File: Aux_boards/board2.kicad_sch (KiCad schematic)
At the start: 30 parts, among them J1 DA15_Plug_MountingHoles, U2 AMS1117-3.3, U3 SFH6345, U4 SFH6345, U5 SFH6345, U6 SFH6345, U7 SFH6345, U8 SFH6345, U9 SFH6345

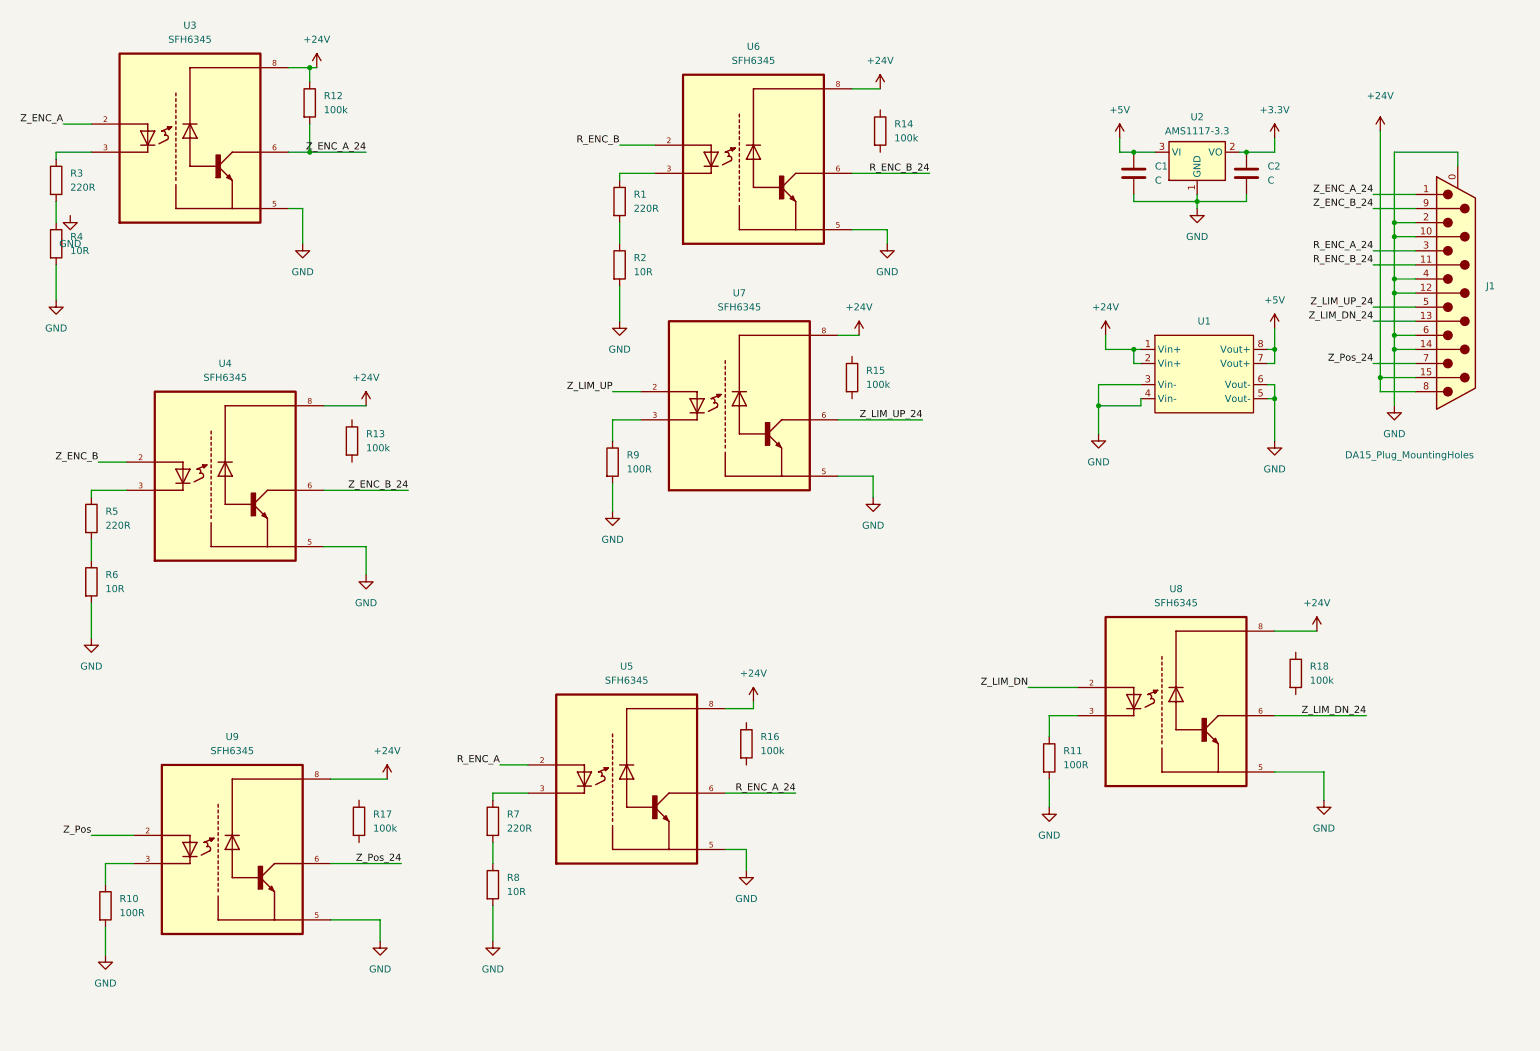
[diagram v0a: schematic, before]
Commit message: jeee
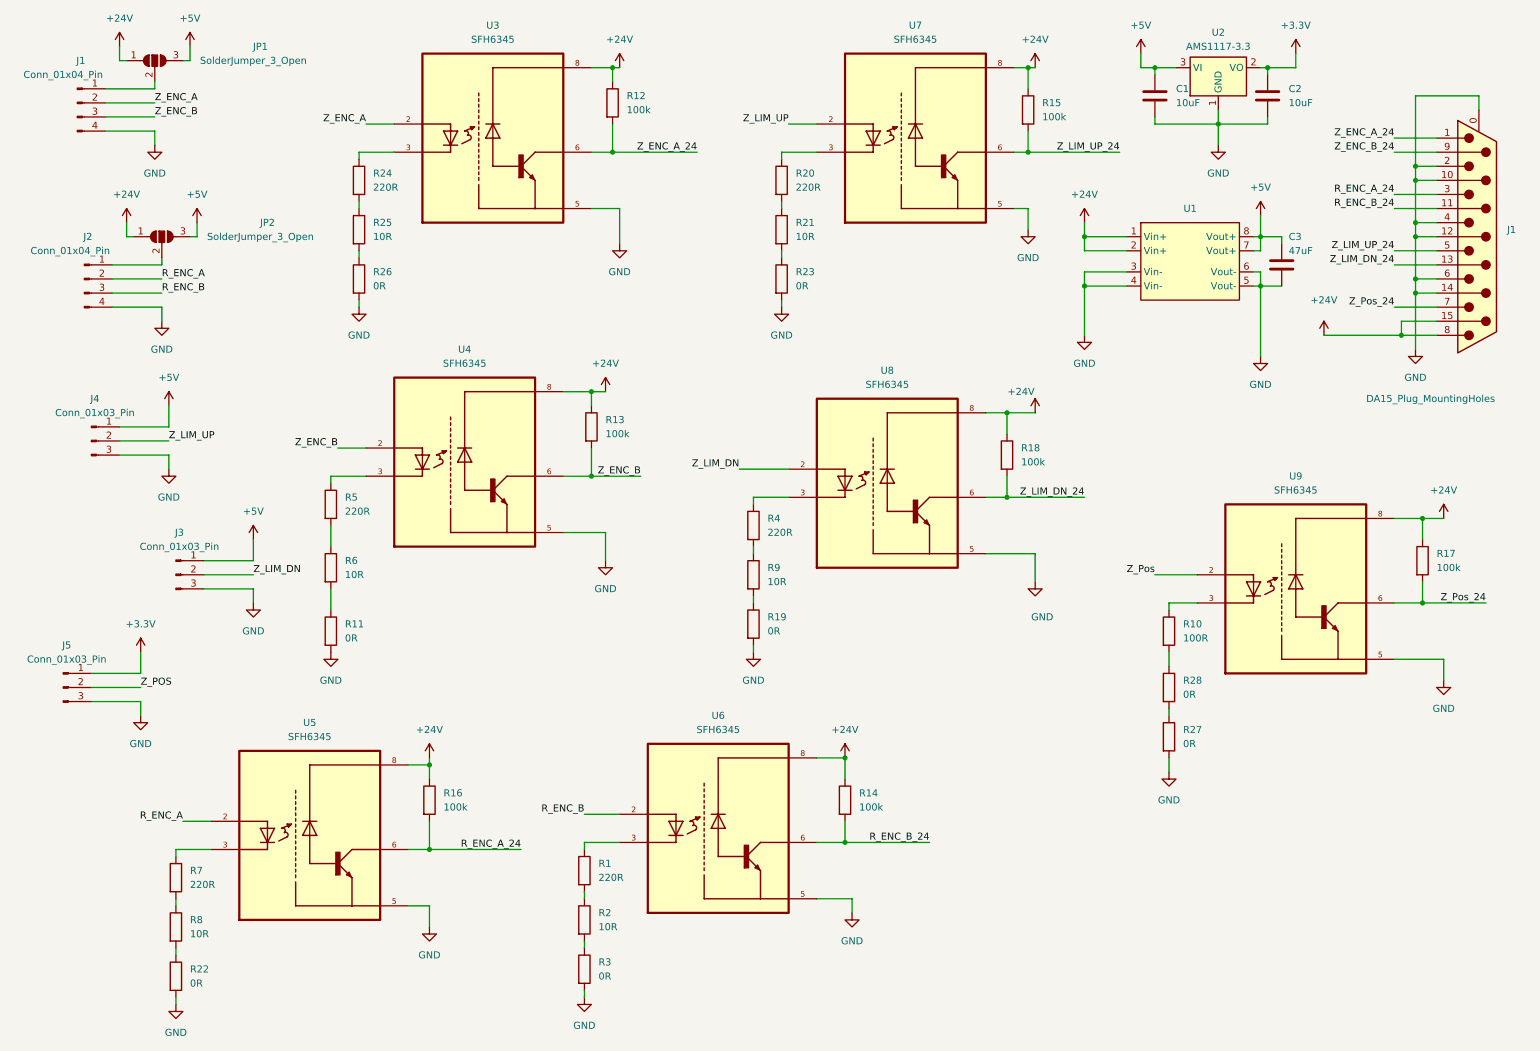
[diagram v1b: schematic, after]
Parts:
- added C3: 47uF, symbol Device:C
- added J1, J2: Conn_01x04_Pin, symbol Connector:Conn_01x04_Pin
- added J3, J4, J5: Conn_01x03_Pin, symbol Connector:Conn_01x03_Pin
- added JP1, JP2: SolderJumper_3_Open, symbol Jumper:SolderJumper_3_Open
- added R19, R22, R23, R26, R27, R28: 0R, symbol Device:R
- added R20, R24: 220R, symbol Device:R
- added R21, R25: 10R, symbol Device:R
- C1, C2: value C -> 10uF
- R11: value 100R -> 0R
- R3: value 220R -> 0R
- R4: value 10R -> 220R
- R9: value 100R -> 10R
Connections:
- net +24V: now also R13.1, R14.1, R15.1, R16.1, R17.1, R18.1, JP1.1 (A), JP2.1 (A)
- net +3.3V: now also J5.1 (Pin_1)
- net +5V: now also C3.1, J3.1 (Pin_1), J4.1 (Pin_1), JP1.3 (B), JP2.3 (B)
- net GND: now also R3.2, C3.2, J1.4 (Pin_4), J2.4 (Pin_4), J3.3 (Pin_3), J4.3 (Pin_3), J5.3 (Pin_3), R19.2, R22.2, R23.2, R26.2, R27.2; no longer R10.2, R2.2, R4.2, R6.2, R8.2, R9.2
- net R_ENC_A: now also J2.2 (Pin_2)
- net R_ENC_A_24: now also R16.2
- net R_ENC_B: now also J2.3 (Pin_3)
- net R_ENC_B_24: now also R14.2
- net Z_ENC_A: now also J1.2 (Pin_2)
- net Z_ENC_B: now also R13.2, U4.6, J1.3 (Pin_3)
- net Z_ENC_B_24: no longer U4.6
- net Z_LIM_DN: now also J3.2 (Pin_2)
- net Z_LIM_DN_24: now also R18.2
- net Z_LIM_UP: now also J4.2 (Pin_2)
- net Z_LIM_UP_24: now also R15.2
- net Z_Pos_24: now also R17.2
- net at U8.3: now also R4.1; no longer R11.1
- net at U7.3: now also R20.1; no longer R9.1
- net at R3.1: now also R2.2; no longer U3.3
- new net: R20.2, R21.1
- new net: J2.1 (Pin_1), JP2.2 (C)
- new net: R10.2, R28.1
- new net: R22.1, R8.2
- new net: R11.1, R6.2
- new net: R4.2, R9.1
- new net: J1.1 (Pin_1), JP1.2 (C)
- new net: R24.1, U3.3
- new net: R21.2, R23.1
- new net: R27.1, R28.2
- new net: R24.2, R25.1
- new net: R25.2, R26.1
- new net: R19.1, R9.2
- new net Z_POS: J5.2 (Pin_2)
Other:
- company: (none) -> LEGO Kör (legokor.hu)
- title: (none) -> Karcsi (INDACT Robot Arm) - Aux. control board II.
- moved on the sheet: C1, C2, J1, R10, R12, R13, R14, R15, R16, R17, R18, R5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
